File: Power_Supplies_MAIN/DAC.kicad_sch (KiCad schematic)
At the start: 51 parts, among them J1 Line Out (Left), J2 Headphone Out, J21 Line Out (Right), J33 PINHD_1x3_Female, J36 PINHD_1x2_Female, U10 OPA2134, U11 TPA6110A2DGN, U34 NE5532AD, U35 NE5532AD, U9 PCM1780

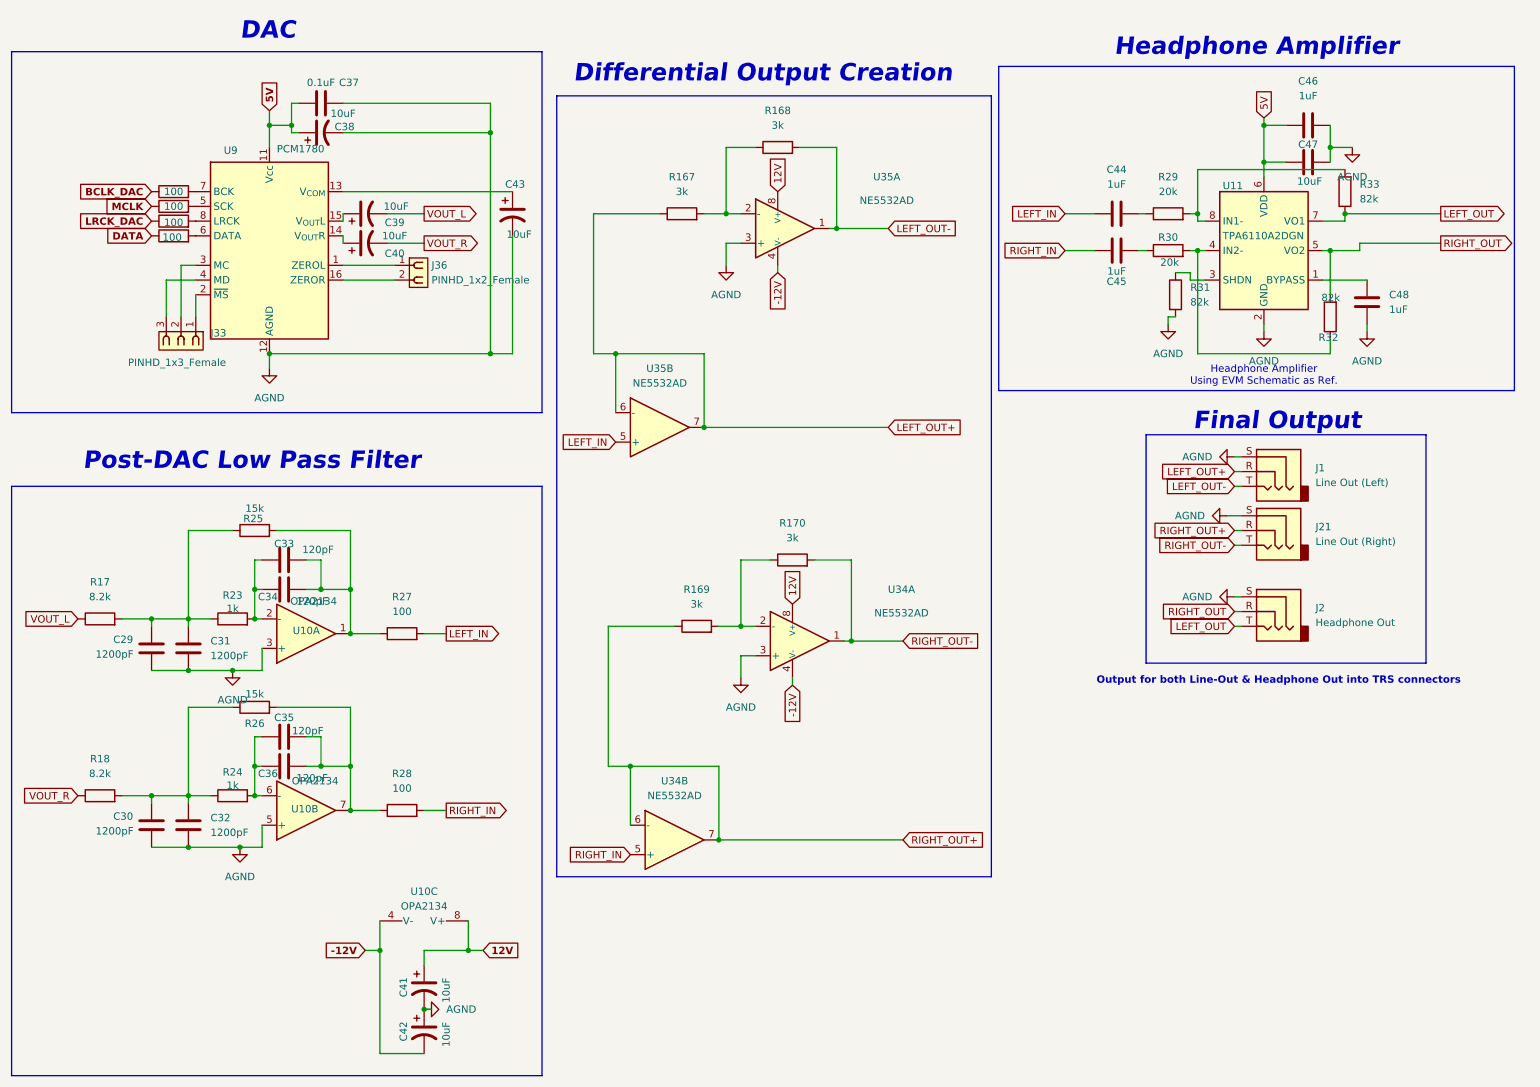
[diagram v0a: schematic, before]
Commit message: fixed a lot of stuff
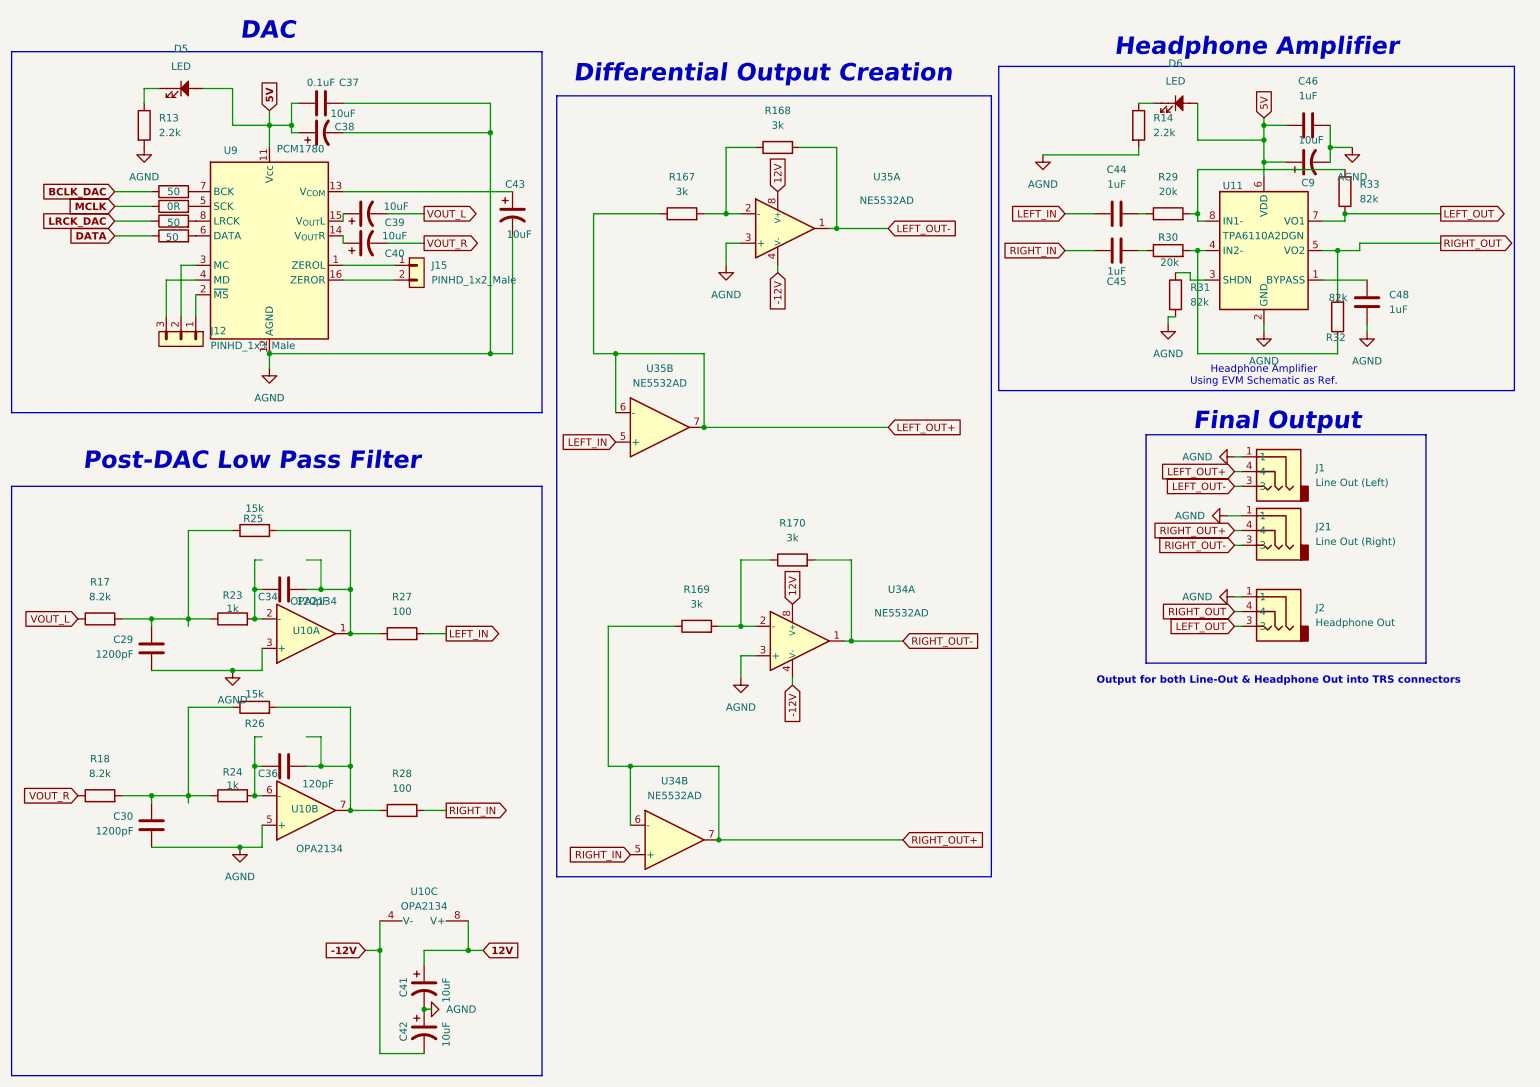
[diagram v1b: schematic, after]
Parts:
- removed C31, C32: 1200pF, Capacitor_SMD:C_0603_1608Metric_Pad1.08x0.95mm_HandSolder, symbol Device:C
- removed C33, C35: 120pF, Capacitor_SMD:C_0603_1608Metric_Pad1.08x0.95mm_HandSolder, symbol Device:C
- removed C47: 10uF, Capacitor_SMD:C_0805_2012Metric, symbol Device:C
- removed J33: PINHD_1x3_Female, Connector_PinSocket_2.54mm:PinSocket_1x03_P2.54mm_Vertical, symbol PCM_SL_Pin_Headers:PINHD_1x3_Female
- removed J36: PINHD_1x2_Female, Connector_PinSocket_2.54mm:PinSocket_1x02_P2.54mm_Vertical, symbol PCM_SL_Pin_Headers:PINHD_1x2_Female
- added C9: 10uF, Capacitor_SMD:CP_Elec_4x5.8, symbol Device:C_Polarized_US
- added D5, D6: LED, LED_SMD:LED_0402_1005Metric_Pad0.77x0.64mm_HandSolder, symbol PCM_SL_Devices:LED
- added J12: PINHD_1x3_Male, Connector_PinHeader_2.54mm:PinHeader_1x03_P2.54mm_Vertical, symbol PCM_SL_Pin_Headers:PINHD_1x3_Male
- added J15: PINHD_1x2_Male, Connector_PinHeader_2.54mm:PinHeader_1x02_P2.54mm_Vertical, symbol PCM_SL_Pin_Headers:PINHD_1x2_Male
- added R13, R14: 2.2k, Resistor_SMD:R_0805_2012Metric, symbol Device:R
- J1, J2, J21: footprint Connector_Audio:Jack_3.5mm_CUI_SJ-3523-SMT_Horizontal -> SamacSys_Parts:ACJSNV353
- R19, R21, R22: value 100 -> 50
- R20: value 100 -> 0R
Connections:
- net 5V: now also C9.1, D5.2, D6.2
- net AGND: now also J1.1, J2.1, J21.1, C9.2, R13.2, R14.2; no longer J1.S, J2.S, J21.S
- net LEFT_OUT: now also J2.3; no longer J2.T
- net LEFT_OUT+: now also J1.4; no longer J1.R
- net LEFT_OUT-: now also J1.3; no longer J1.T
- net RIGHT_OUT: now also J2.4; no longer J2.R
- net RIGHT_OUT+: now also J21.4; no longer J21.R
- net RIGHT_OUT-: now also J21.3; no longer J21.T
- net at U9.2 (~{MS}): now also J12.1
- net at U9.3 (MC): now also J12.2
- net at U9.4 (MD): now also J12.3
- net at U9.1 (ZEROL): now also J15.1
- net at U9.16 (ZEROR): now also J15.2
- new net: D5.1, R13.1
- new net: D6.1, R14.1
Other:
- moved on the sheet: R32
